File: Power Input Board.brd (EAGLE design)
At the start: 136.7 x 125.3 mm, 19 parts, among them Q1 SPB80P06P

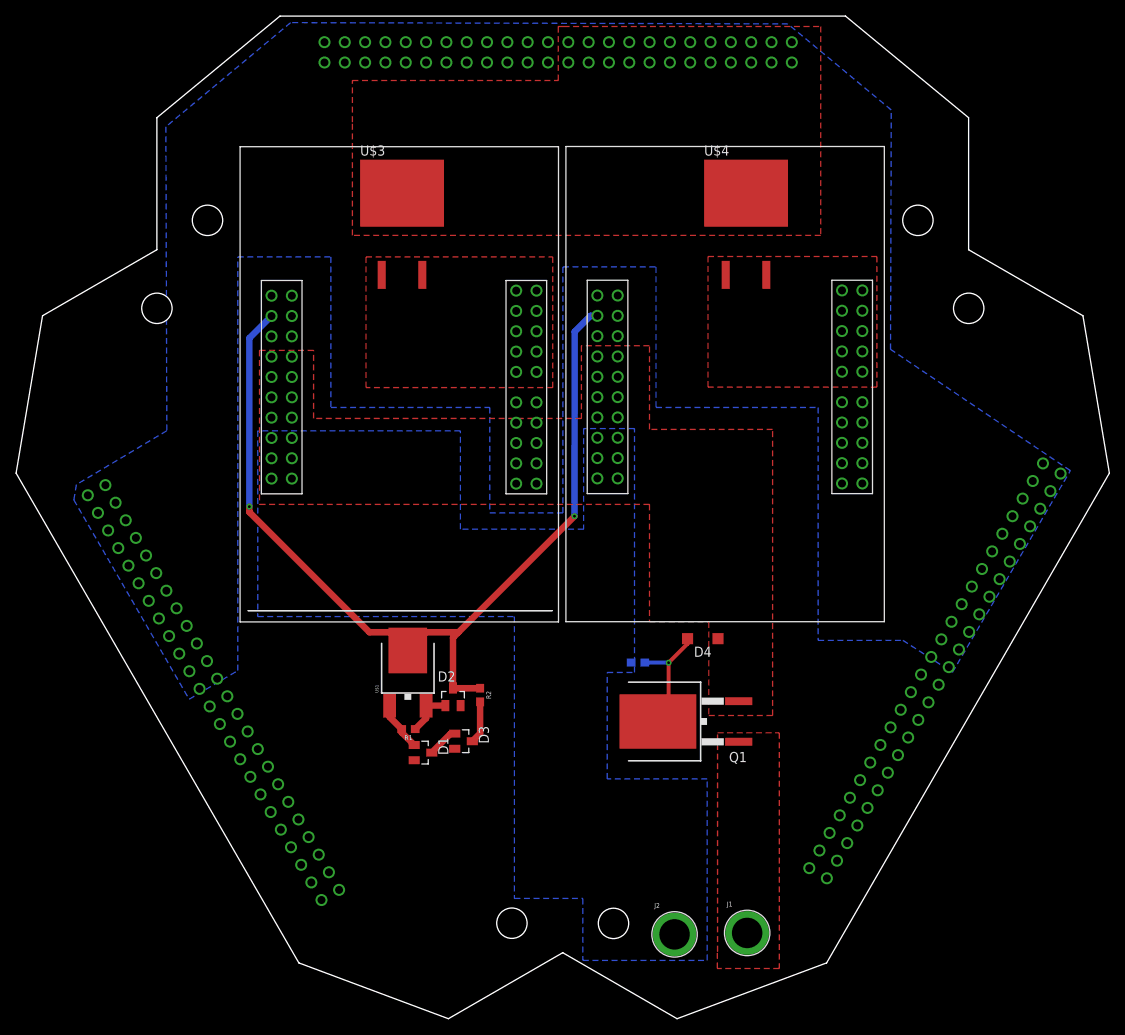
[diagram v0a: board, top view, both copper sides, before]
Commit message: fixed some stuff
moved things around
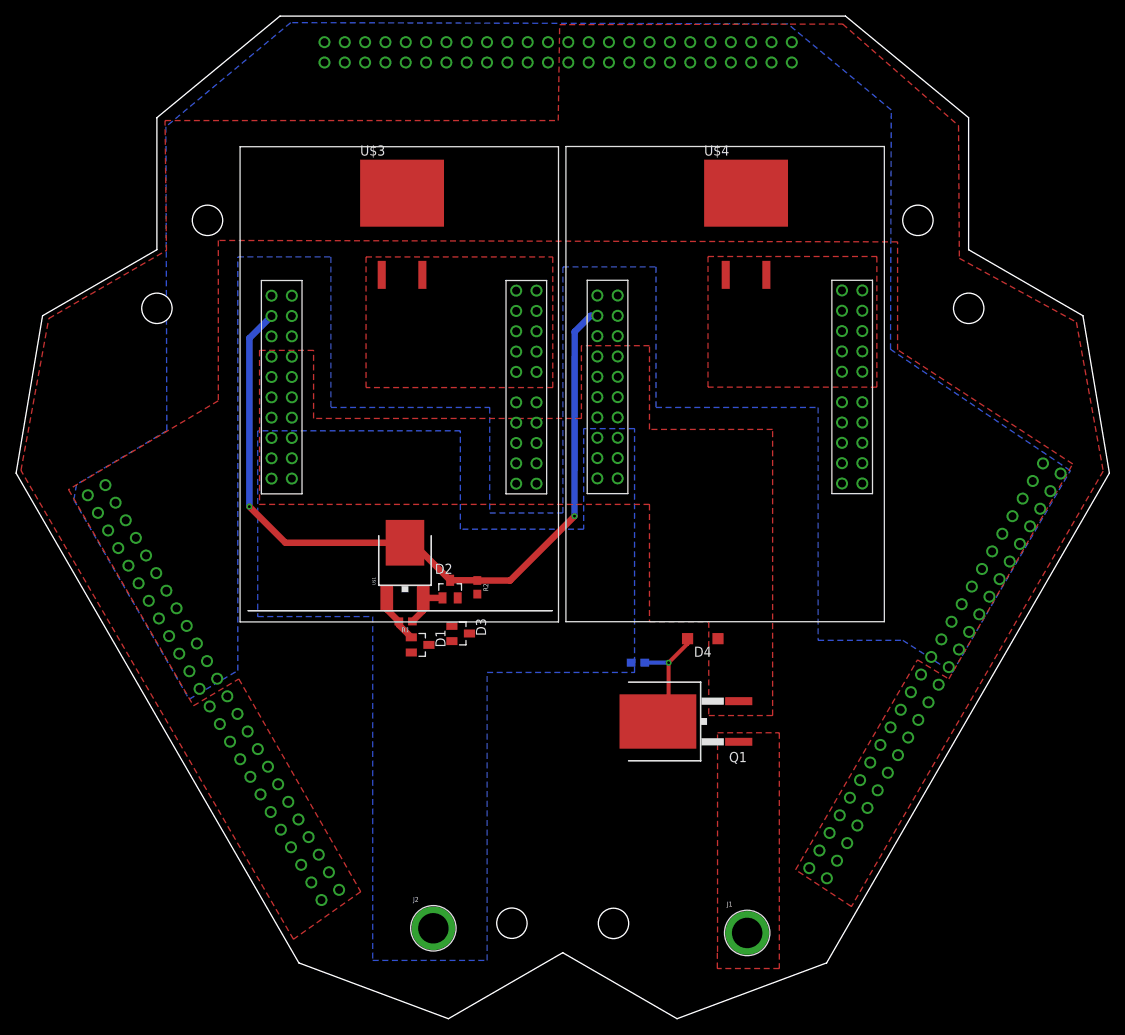
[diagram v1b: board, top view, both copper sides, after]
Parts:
- moved J2 30.2 mm to (52.2, 11.3)
- moved D2 13.5 mm to (54.3, 53.7)
- moved D3 13.5 mm to (55.6, 48.1)
- moved R2 13.5 mm to (57.7, 53.9)
- moved U$1 13.5 mm to (48.6, 57.9)
- moved D1 13.5 mm to (50.5, 46.7)
- moved R1 13.5 mm to (48.7, 49.7)
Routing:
- net ON/OFF: track 117.9 -> 99.6 mm
- net N$5: track 5.33 -> 0.00 mm
- net N$1: track 3.85 -> 0.00 mm
